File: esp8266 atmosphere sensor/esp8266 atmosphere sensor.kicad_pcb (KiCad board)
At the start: 4 copper layers, 52.7 x 47.6 mm, 61 parts, among them J1 Conn_02x03_Odd_Even, J10 Conn_01x03, J11 Conn_01x03, J12 Conn_01x03, J13 Conn_01x03, J14 Conn_01x03, J2 UJ2-MIBH-G-SMT-TR, J3 LUX sensor, J4 bme280, J5 PIR, J6 Analog in, J7 external i2c, J8 power, J9 Conn_01x03, SW1 SW_MEC_5E, U1 ESP-12F, U2 LD1117S33

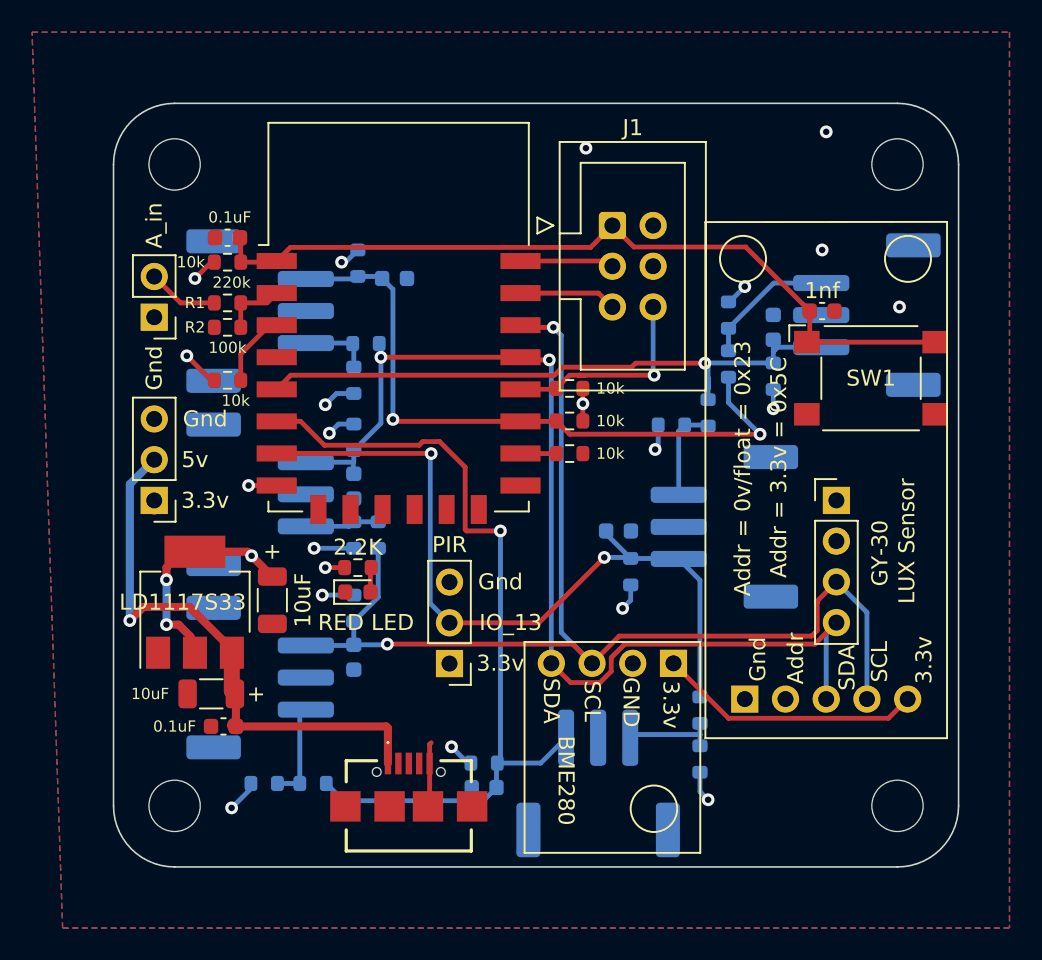
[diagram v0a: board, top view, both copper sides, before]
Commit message: generated gerbers, added gitignore
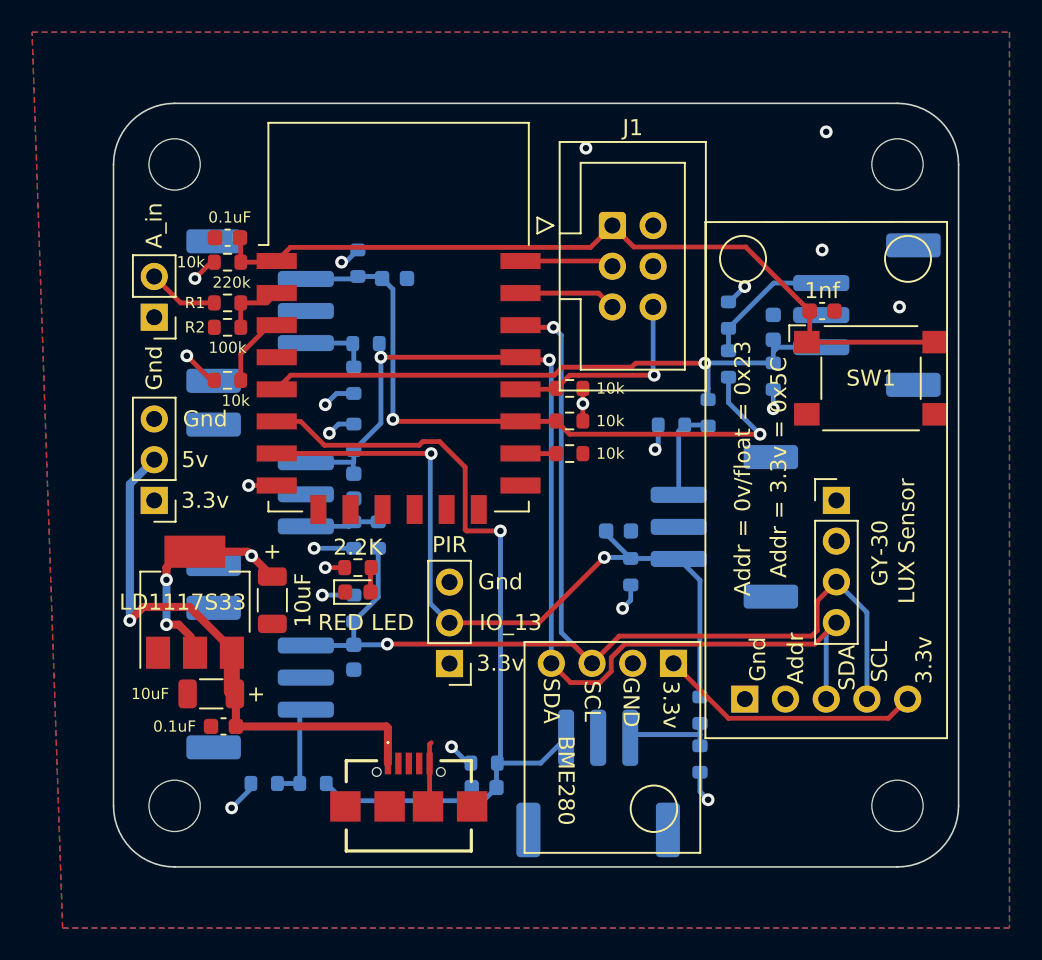
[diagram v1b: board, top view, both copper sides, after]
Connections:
- J10 pad MP: GND -> (no net)
- J11 pad MP: GND -> (no net)
- J12 pad MP: GND -> (no net)
- J13 pad MP: GND -> (no net)
- J14 pad MP: GND -> (no net)
- J9 pad MP: GND -> (no net)
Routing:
- net +3V3: track 49.1 -> 48.1 mm
- net /ESP_IO14: track 39.2 -> 38.6 mm
